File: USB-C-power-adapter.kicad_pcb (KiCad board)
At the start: 2 copper layers, 21.1 x 40.1 mm, 80 parts, among them J1 JST_SH_1x4_SM04B-SRSS-TB-LF-SN, J2 Molex_Nano-Fit_1x2_105313-220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, J3 USB-C_GCT_USB4105-GF-A, J4 JST_SH_1x4_SM04B-SRSS-TB-LF-SN, Q1 SQS401EN-T1_BE3, U1 TPD4E02B04DQA, U2 TPD4E02B04DQA, U3 STUSB4500_QFN, U4 SIC477ED-T1-GE3, U5 AP62301WU-7, U6 AP62301WU-7

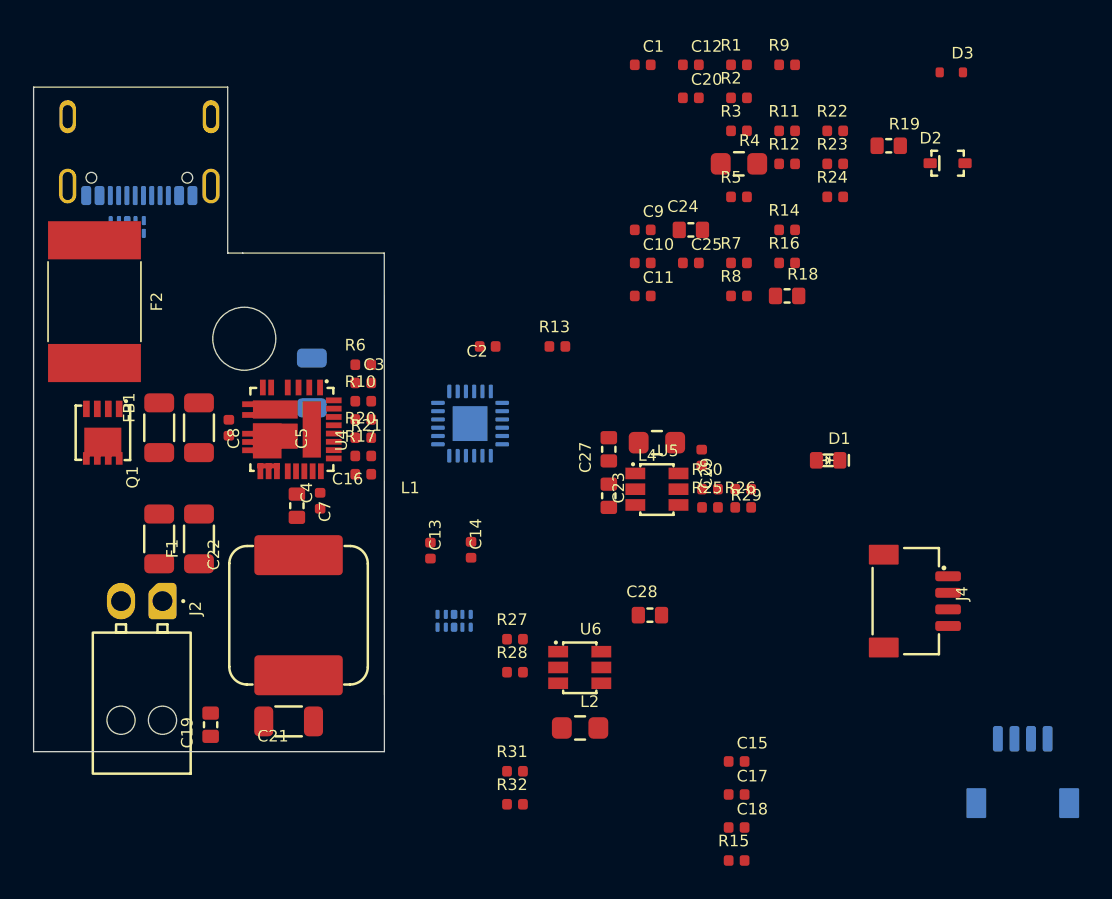
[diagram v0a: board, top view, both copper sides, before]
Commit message: [#57225] Placement
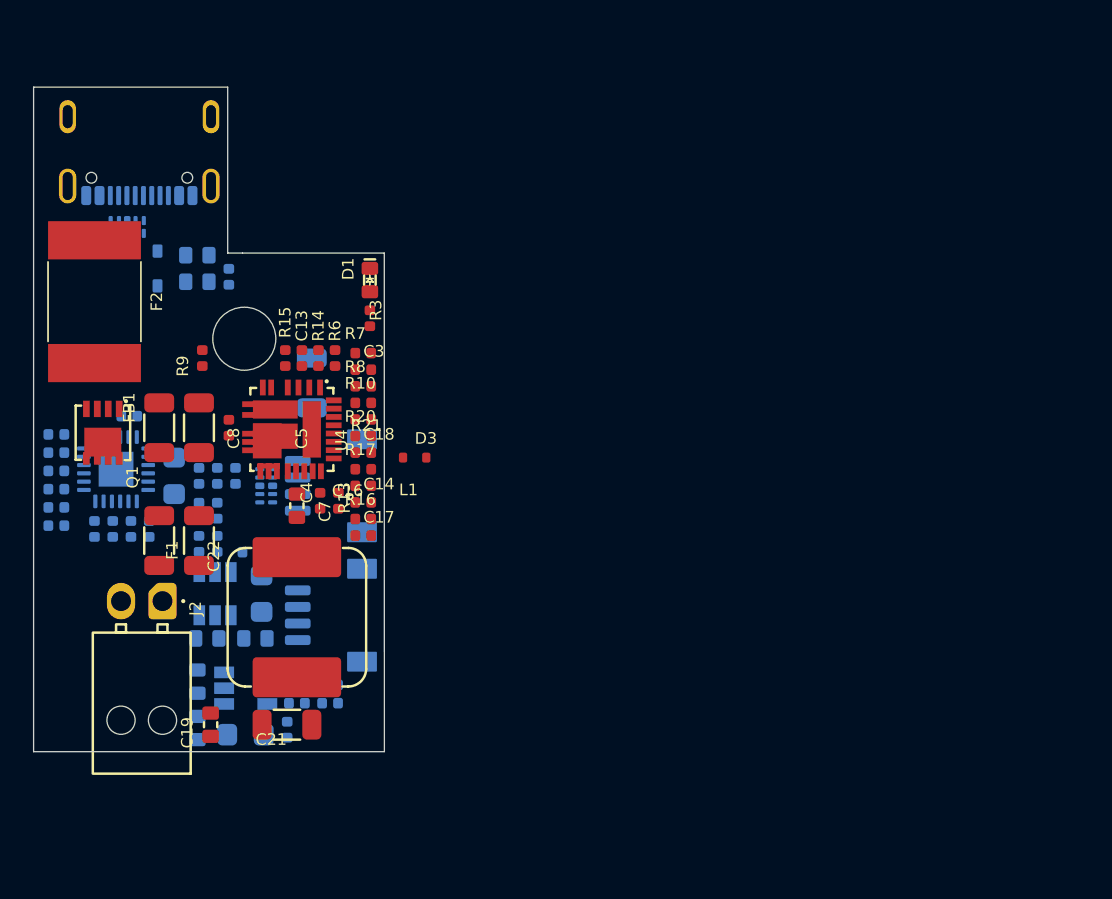
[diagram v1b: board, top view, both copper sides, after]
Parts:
- C1, C10, C11, C12, C15, C2, C20, C23, C24, C25, C27, C28, C29, C9, D2, J4, L2, L4, R1, R11, R12, R18, R19, R2, R22, R23, R24, R25, R26, R27, R28, R29, R30, R31, R32, R4, R5, U5, U6: moved to B.Cu
- moved R12 49.1 mm to (82.9, 87.5), turned to 180 degrees
- moved R11 49.1 mm to (82.9, 85.3)
- moved D2 48.0 mm to (89.0, 72.0), turned to 90 degrees
- moved R24 47.9 mm to (86.3, 87.7), turned to 90 degrees
- moved R23 47.8 mm to (87.4, 87.7), turned to -90 degrees
- moved R22 47.8 mm to (88.5, 87.7), turned to 90 degrees
- moved J1 44.9 mm to (99.9, 85.1), turned to -90 degrees
- moved C20 44.4 mm to (85.2, 87.7), turned to -90 degrees
- moved C12 44.3 mm to (82.9, 82.0)
- moved R19 42.5 mm to (91.4, 72.8)
- moved C15 42.3 mm to (93.3, 72.5), turned to 90 degrees
- moved R15 40.7 mm to (96.7, 77.4), turned to -90 degrees
- moved R1 40.0 mm to (92.6, 84.5), turned to 90 degrees
- moved D3 39.8 mm to (104.5, 83.4)
- moved R2 39.7 mm to (91.5, 84.5), turned to 90 degrees
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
